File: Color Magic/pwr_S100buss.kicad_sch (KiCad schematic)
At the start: 39 parts, among them P1 S100_MALE, U14 LM7805K, U49 LM78L12

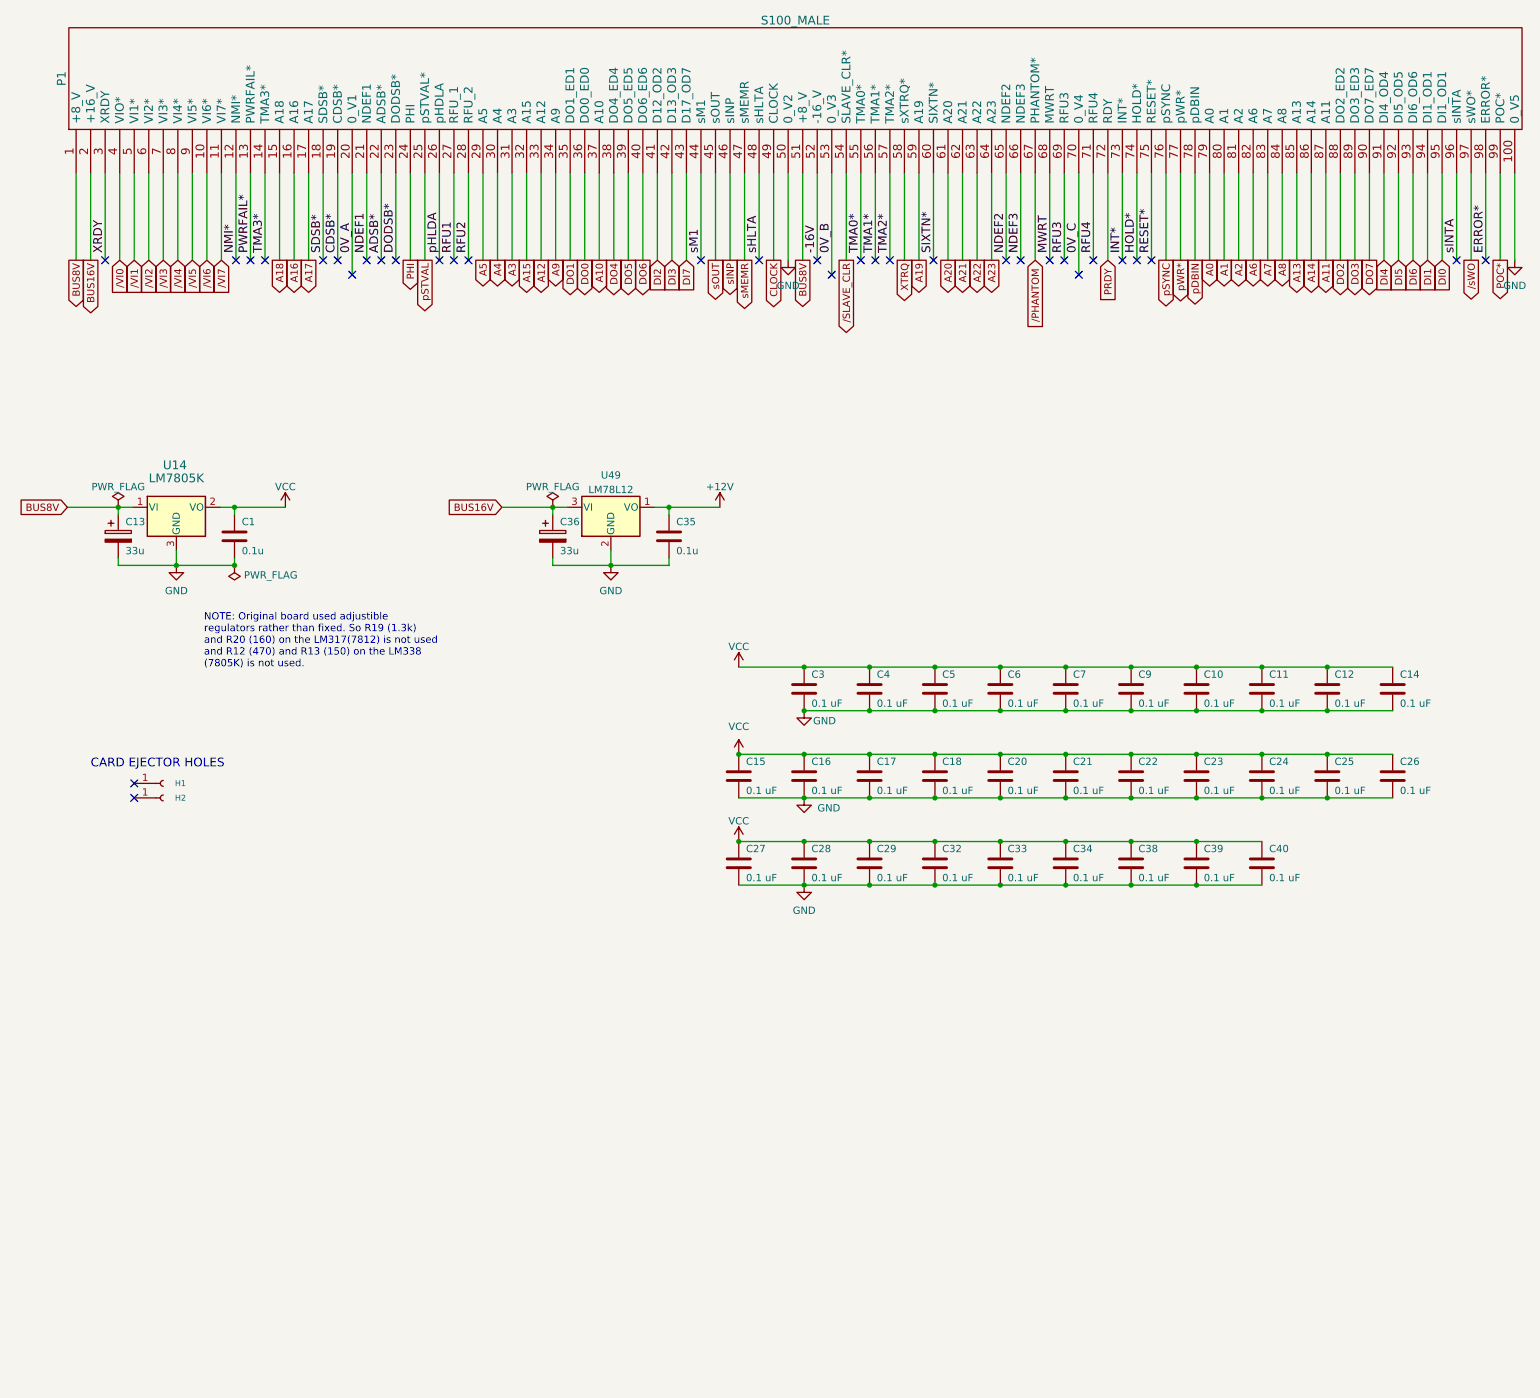
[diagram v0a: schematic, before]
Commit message: Add files via upload
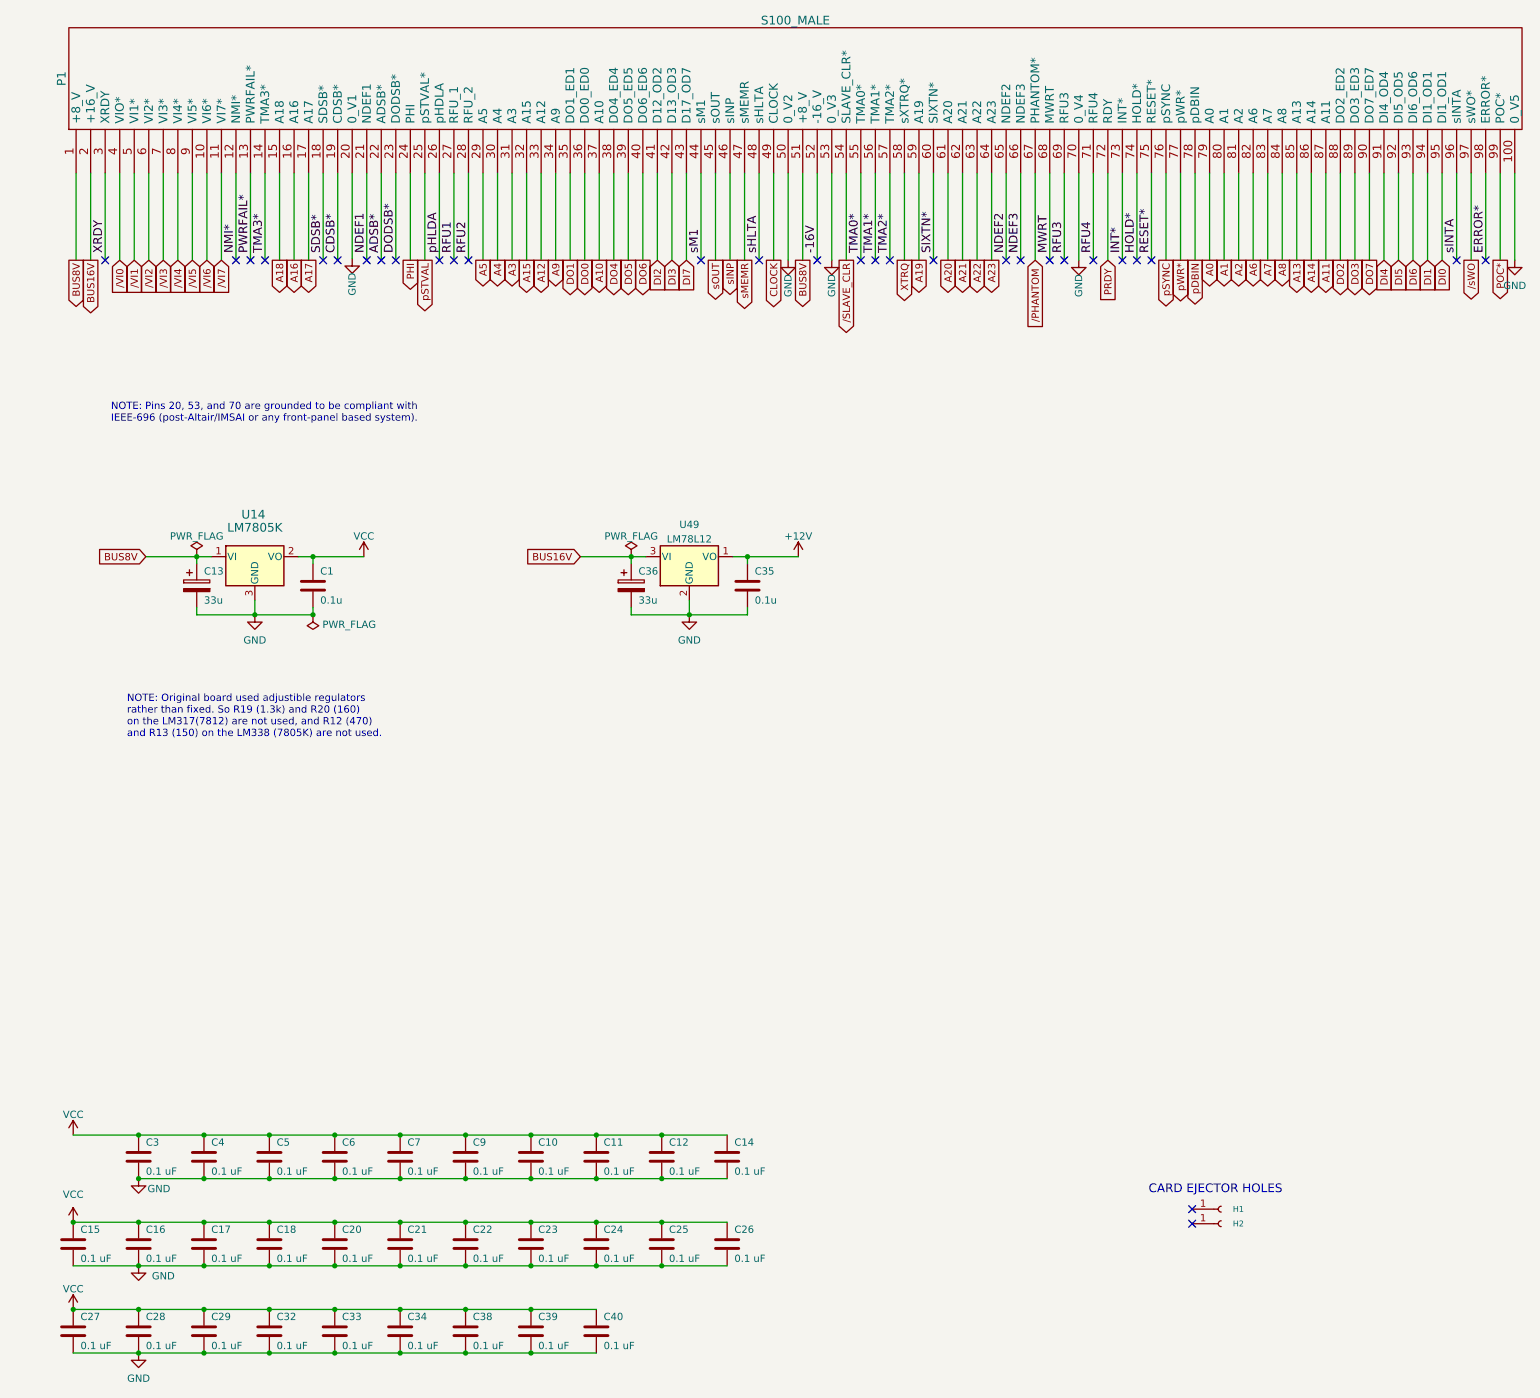
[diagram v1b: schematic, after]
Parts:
- P1: symbol RAC_Custom2:S100_MALE -> RAC_Custom:S100_MALE
- U14: symbol RAC_Custom2:LM7805K -> RAC_Custom:LM7805K
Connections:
- net 0V_A is gone; now on net GND: P1.20 (0_V1)
- net 0V_B is gone; now on net GND: P1.53 (0_V3)
- net 0V_C is gone; now on net GND: P1.70 (0_V4)
- no-connect marks 34 -> 31
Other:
- note added: "NOTE: Original board used adjustible regulators rather than fixed. So R19 (1.3k) and R20 (160) on the LM317(7812) are not used, and R12 (470) and R13 (150) on the LM338 (7805K) are not used."
- note added: "NOTE: Pins 20, 53, and 70 are grounded to be compliant with IEEE-696 (post-Altair/IMSAI or any front-panel based system)."
- note removed: "NOTE: Original board used adjustible regulators rather than fixed. So R19 (1.3k) and R20 (160) on the LM317(7812) is not used and R12 (470) and R13 (150) on the LM338 (7805K) is not used."
- moved on the sheet: C1, C10, C11, C12, C13, C14, C15, C16, C17, C18, C20, C21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
